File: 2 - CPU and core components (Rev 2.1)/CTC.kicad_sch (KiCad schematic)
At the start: 2 parts

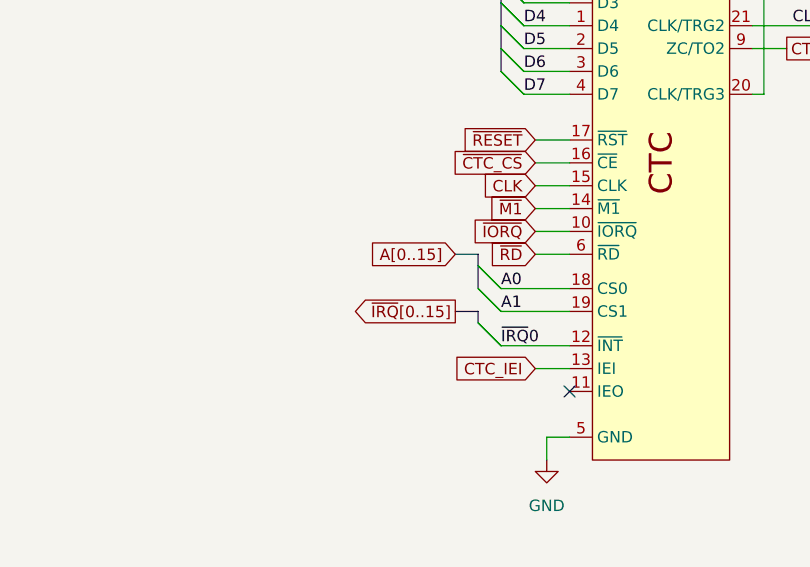
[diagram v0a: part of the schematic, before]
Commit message: Trying to work out the PLD logic
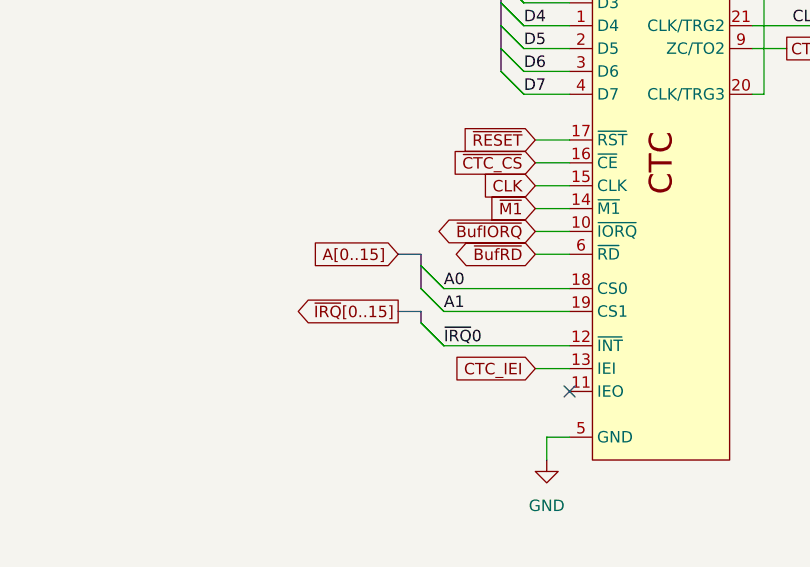
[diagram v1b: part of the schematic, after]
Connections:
- net ~{IORQ} renamed ~{BufIORQ}
- net ~{RD} renamed ~{BufRD}
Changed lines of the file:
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@@
     (stroke (width 0) (type default))
   )
-  (bus_entry (at 118.11 115.57) (size 2.54 2.54)
-    (stroke (width 0) (type default))
-  )
-  (bus_entry (at 118.11 109.22) (size 2.54 2.54)
+  (bus_entry (at 111.76 115.57) (size 2.54 2.54)
+    (stroke (width 0) (type default))
+  )
+  (bus_entry (at 111.76 109.22) (size 2.54 2.54)
     (stroke (width 0) (type default))
   )
@@
     (stroke (width 0) (type default))
   )
-  (bus_entry (at 118.11 115.57) (size 2.54 2.54)
+  (bus_entry (at 111.76 115.57) (size 2.54 2.54)
     (stroke (width 0) (type default))
   )
@@
     (stroke (width 0) (type default))
   )
-  (bus_entry (at 118.11 111.76) (size 2.54 2.54)
+  (bus_entry (at 111.76 111.76) (size 2.54 2.54)
     (stroke (width 0) (type default))
   )
@@
     (stroke (width 0) (type default))
   )
-  (bus_entry (at 118.11 109.22) (size 2.54 2.54)
+  (bus_entry (at 111.76 109.22) (size 2.54 2.54)
     (stroke (width 0) (type default))
   )
@@
     (stroke (width 0) (type default))
   )
-  (bus_entry (at 118.11 111.76) (size 2.54 2.54)
+  (bus_entry (at 111.76 111.76) (size 2.54 2.54)
     (stroke (width 0) (type default))
   )
@@
     (stroke (width 0) (type default))
   )
-  (wire (pts (xy 120.65 111.76) (xy 128.27 111.76))
-    (stroke (width 0) (type default))
-  )
   (wire (pts (xy 124.46 120.65) (xy 128.27 120.65))
     (stroke (width 0) (type default))
   )
-  (bus (pts (xy 118.11 115.57) (xy 118.11 114.3))
+  (bus (pts (xy 111.76 115.57) (xy 111.76 114.3))
     (stroke (width 0) (type default))
   )
@@
     (stroke (width 0) (type default))
   )
+  (wire (pts (xy 114.3 111.76) (xy 128.27 111.76))
+    (stroke (width 0) (type default))
+  )
   (wire (pts (xy 125.73 128.27) (xy 125.73 130.81))
     (stroke (width 0) (type default))
@@
     (stroke (width 0) (type default))
   )
-  (bus (pts (xy 115.57 114.3) (xy 118.11 114.3))
+  (bus (pts (xy 109.22 114.3) (xy 111.76 114.3))
     (stroke (width 0) (type default))
   )
@@
     (stroke (width 0) (type default))
   )
-  (wire (pts (xy 120.65 118.11) (xy 128.27 118.11))
+  (wire (pts (xy 114.3 118.11) (xy 128.27 118.11))
     (stroke (width 0) (type default))
   )
@@
     (stroke (width 0) (type default))
   )
-  (bus (pts (xy 118.11 109.22) (xy 118.11 107.95))
+  (bus (pts (xy 111.76 109.22) (xy 111.76 107.95))
     (stroke (width 0) (type default))
   )
@@
     (stroke (width 0) (type default))
   )
-  (bus (pts (xy 118.11 111.76) (xy 118.11 109.22))
+  (bus (pts (xy 111.76 111.76) (xy 111.76 109.22))
     (stroke (width 0) (type default))
   )
@@
     (stroke (width 0) (type default))
   )
-  (bus (pts (xy 115.57 107.95) (xy 118.11 107.95))
+  (bus (pts (xy 109.22 107.95) (xy 111.76 107.95))
     (stroke (width 0) (type default))
   )
@@
     (stroke (width 0) (type default))
   )
-  (wire (pts (xy 120.65 114.3) (xy 128.27 114.3))
+  (wire (pts (xy 114.3 114.3) (xy 128.27 114.3))
     (stroke (width 0) (type default))
   )
@@
     (effects (font (size 1.27 1.27)) (justify left bottom))
   )
-  (label "A0" (at 120.65 111.76 0) (fields_autoplaced)
+  (label "A0" (at 114.3 111.76 0) (fields_autoplaced)
     (effects (font (size 1.27 1.27)) (justify left bottom))
   )
@@
     (effects (font (size 1.27 1.27)) (justify left bottom))
   )
-  (label "~{IRQ}0" (at 120.65 118.11 0) (fields_autoplaced)
+  (label "~{IRQ}0" (at 114.3 118.11 0) (fields_autoplaced)
     (effects (font (size 1.27 1.27)) (justify left bottom))
   )
@@
     (effects (font (size 1.27 1.27)) (justify right bottom))
   )
-  (label "A1" (at 120.65 114.3 0) (fields_autoplaced)
+  (label "A1" (at 114.3 114.3 0) (fields_autoplaced)
     (effects (font (size 1.27 1.27)) (justify left bottom))
   )
@@
   (label "D2" (at 123.19 77.47 0) (fields_autoplaced)
     (effects (font (size 1.27 1.27)) (justify left bottom))
-  )
-  (global_label "~{IORQ}" (shape input) (at 124.46 105.41 180) (fields_autoplaced)
-    (effects (font (size 1.27 1.27)) (justify right))
-    (property "Intersheetrefs" "${INTERSHEET_REFS}" (at 116.939 105.41 0)
-      (effects (font (size 1.27 1.27)) (justify right) hide)
-    )
   )
   (global_label "CLK" (shape input) (at 124.46 100.33 180) (fields_autoplaced)
@@
     )
   )
-  (global_label "~{RD}" (shape input) (at 124.46 107.95 180) (fields_autoplaced)
-    (effects (font (size 1.27 1.27)) (justify right))
-    (property "Intersheetrefs" "${INTERSHEET_REFS}" (at 118.9348 107.95 0)
-      (effects (font (size 1.27 1.27)) (justify right) hide)
-    )
-  )
   (global_label "CTCLK0" (shape output) (at 152.4 77.47 0) (fields_autoplaced)
     (effects (font (size 1.27 1.27)) (justify left))
@@
     )
   )
+  (global_label "~{BufIORQ}" (shape tri_state) (at 124.46 105.41 180) (fields_autoplaced)
+    (effects (font (size 1.27 1.27)) (justify right))
+    (property "Intersheetrefs" "${INTERSHEET_REFS}" (at 112.683 105.41 0)
+      (effects (font (size 1.27 1.27)) (justify right) hide)
+    )
+  )
+  (global_label "~{BufRD}" (shape tri_state) (at 124.46 107.95 180) (fields_autoplaced)
+    (effects (font (size 1.27 1.27)) (justify right))
+    (property "Intersheetrefs" "${INTERSHEET_REFS}" (at 114.6788 107.95 0)
+      (effects (font (size 1.27 1.27)) (justify right) hide)
+    )
+  )
   (global_label "D[0..7]" (shape bidirectional) (at 118.11 68.58 180) (fields_autoplaced)
     (effects (font (size 1.27 1.27)) (justify right))
@@
     )
   )
-  (global_label "~{IRQ}[0..15]" (shape output) (at 115.57 114.3 180) (fields_autoplaced)
-    (effects (font (size 1.27 1.27)) (justify right))
-    (property "Intersheetrefs" "${INTERSHEET_REFS}" (at 102.848 114.3 0)
-      (effects (font (size 1.27 1.27)) (justify right) hide)
-    )
-  )
-  (global_label "A[0..15]" (shape input) (at 115.57 107.95 180) (fields_autoplaced)
-    (effects (font (size 1.27 1.27)) (justify right))
-    (property "Intersheetrefs" "${INTERSHEET_REFS}" (at 104.9647 107.95 0)
-      (effects (font (size 1.27 1.27)) (justify right) hide)
-    )
+  (global_label "~{IRQ}[0..15]" (shape output) (at 109.22 114.3 180) (fields_autoplaced)
+    (effects (font (size 1.27 1.27)) (justify right))
+    (property "Intersheetrefs" "${INTERSHEET_REFS}" (at 96.498 114.3 0)
+      (effects (font (size 1.27 1.27)) (justify right) hide)
+    )
+  )
+  (global_label "A[0..15]" (shape input) (at 109.22 107.95 180) (fields_autoplaced)
+    (effects (font (size 1.27 1.27)) (justify right))
+    (property "Intersheetrefs" "${INTERSHEET_REFS}" (at 98.6147 107.95 0)
+      (effects (font (size 1.27 1.27)) (justify right) hide)
+    )
